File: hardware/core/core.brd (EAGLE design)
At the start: 161 x 144.8 mm, 520 parts, among them IC1 MAX481CSA, IC10 MAX481CSA, IC11 MAX481CSA, IC12 MAX481CSA, IC13 MAX481CSA, IC14 MAX481CSA, IC15 MAX481CSA, IC16 MAX481CSA, IC17 MAX481CSA, IC18 MAX481CSA, IC19 MAX481CSA, IC2 LD117AS12TR, IC20 MAX481CSA, IC21 MAX481CSA, IC22 LD117AS12TR, IC23 LD117AS12TR, IC3 MAX481CSA, IC4 MAX481CSA, IC5 MAX481CSA, IC6 MAX481CSA, IC7 MAX481CSA, IC8 MAX481CSA, IC9 MAX481CSA

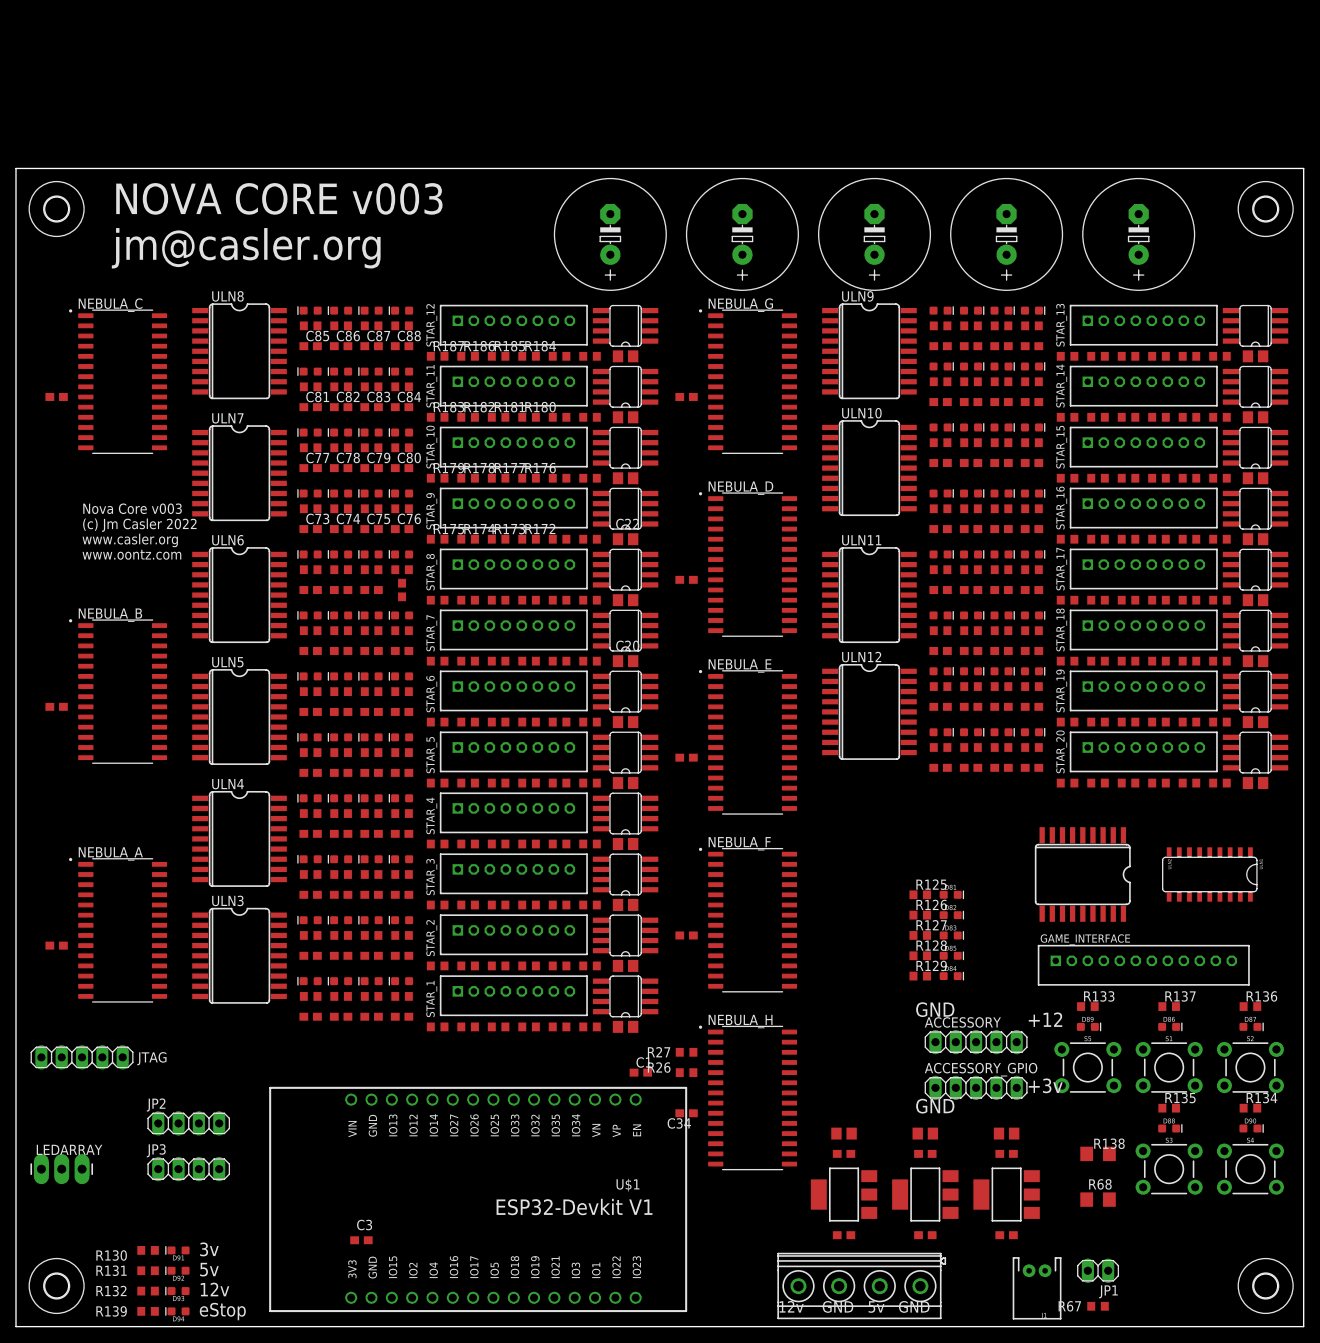
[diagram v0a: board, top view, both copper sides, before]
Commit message: Completed v3
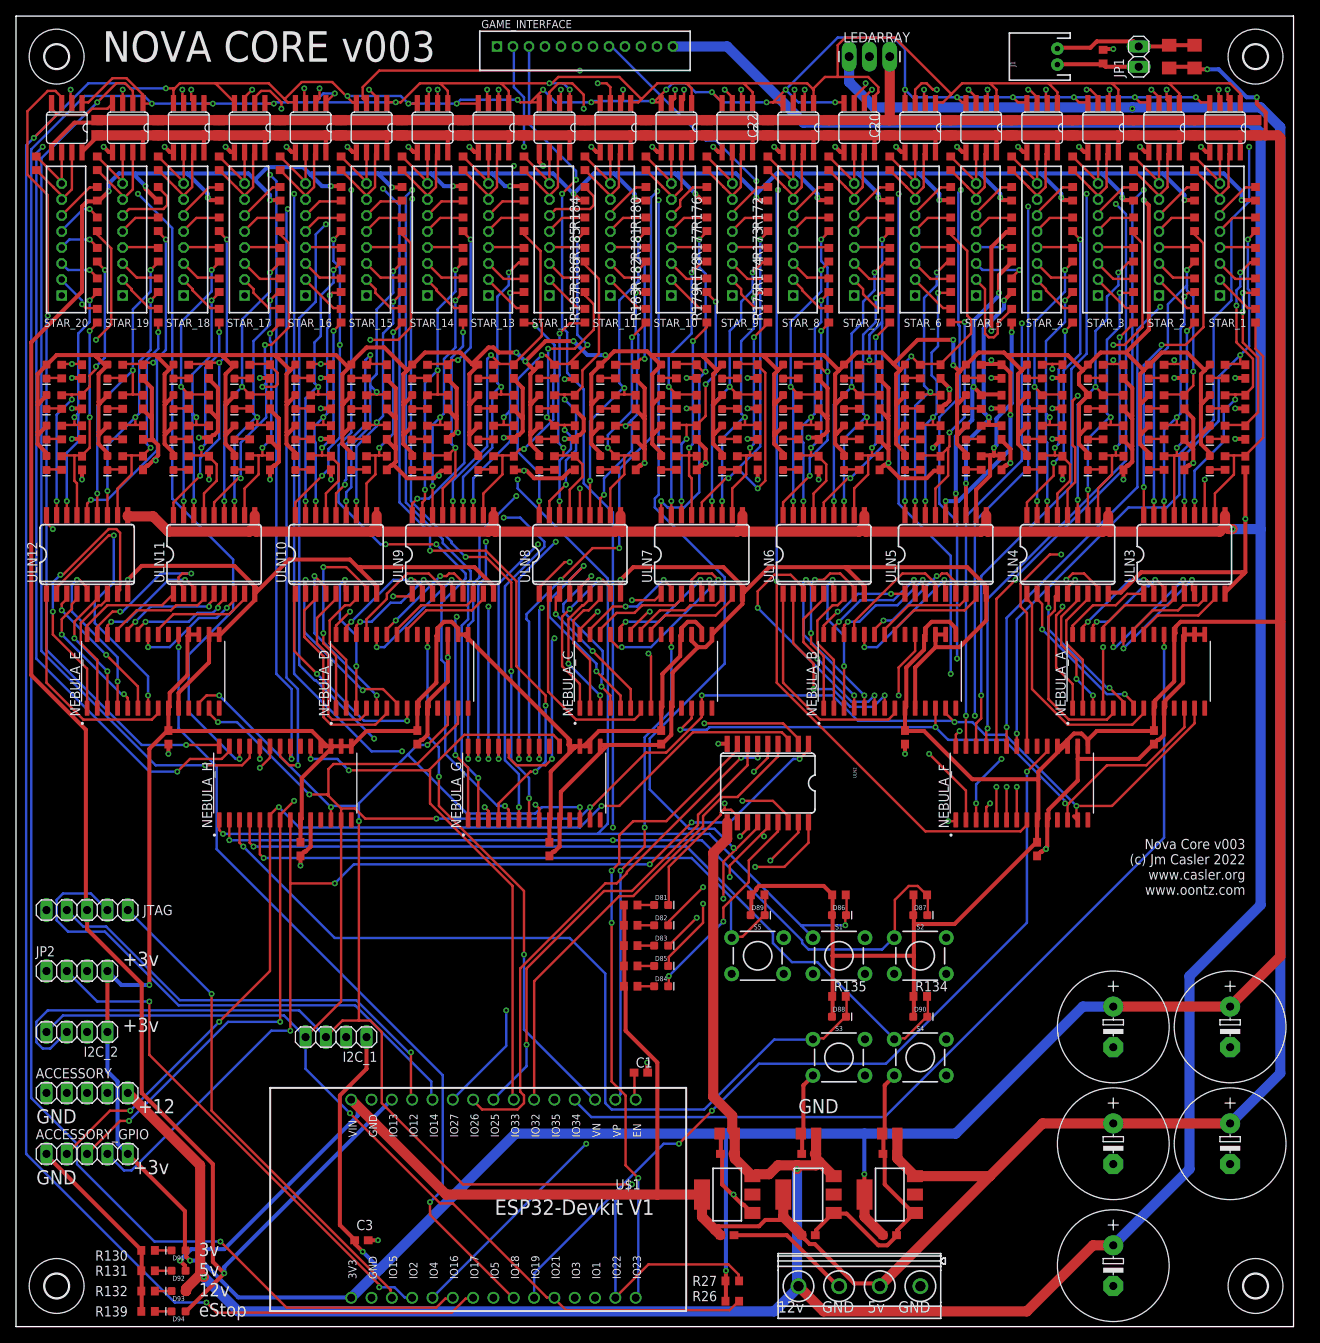
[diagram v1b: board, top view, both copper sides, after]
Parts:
- removed JP3: (no value), pinhead:1X04
- removed ULN1: (no value), SparkFun-IC-Special-Function:SO018
- added I2C_1, I2C_2: (no value), pinhead:1X04
- moved LEDARRAY 171.9 mm to (109.2, 158.8)
- moved IC21 167.9 mm to (6.35, 149.9), turned to 180 degrees
- moved R124 167.0 mm to (2.54, 145.4), turned to 270 degrees
- moved C26 166.3 mm to (10.2, 149.9), turned to 90 degrees
- moved IC20 157.6 mm to (14.0, 149.9), turned to 180 degrees
- moved R123 156.8 mm to (10.2, 145.4), turned to 270 degrees
- moved R67 156.2 mm to (135.9, 158.8), turned to 90 degrees
- moved C27 156.0 mm to (17.8, 149.9), turned to 90 degrees
- moved R106 155.1 mm to (10.2, 141.6), turned to 90 degrees
- moved JP1 151.8 mm to (140.3, 158.8), turned to 90 degrees
- moved J1 151.8 mm to (130.2, 158.8), turned to 90 degrees
- moved R216 150.0 mm to (10.2, 137.8), turned to 90 degrees
- moved STAR_20 149.4 mm to (5.71, 135.9), turned to 90 degrees
- moved IC19 147.4 mm to (21.6, 149.9), turned to 180 degrees
- moved R122 146.6 mm to (17.8, 145.4), turned to 270 degrees
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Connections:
- net +12V: no longer ULN1.10
- net +3V3: now also I2C_1.1, I2C_2.1; no longer JP3.1
- net 21/SDA: now also I2C_1.4, I2C_2.4; no longer JP3.4
- net 22/SCL: now also I2C_1.3, I2C_2.3; no longer JP3.3
- net 23: no longer ULN1.8
- net 25: no longer ULN1.7
- net 26: no longer ULN1.6
- net 27: no longer ULN1.5
- net 32: no longer ULN1.4
- net GND: now also I2C_1.2, I2C_2.2; no longer JP3.2, ULN1.9
- net H13: no longer ULN1.3
- net H14: no longer ULN1.2
- net H15: no longer ULN1.1
- net N$148: no longer ULN1.16
- net N$149: no longer ULN1.17
- net N$150: no longer ULN1.18
- net N$51: no longer ULN1.11
- net N$56: no longer ULN1.12
- net N$57: no longer ULN1.13
- net N$58: no longer ULN1.14
- net N$59: no longer ULN1.15
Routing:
- net +5V: track 0.00 -> 935.7 mm, vias 0 -> 9
- net +3V3: track 0.00 -> 926.9 mm, vias 0 -> 7
- net GND: track 0.00 -> 836.8 mm, vias 0 -> 77
- net +12V: track 0.00 -> 614.6 mm, vias 0 -> 3
- net 13: track 0.00 -> 454.0 mm, vias 0 -> 21
- net 16: track 0.00 -> 413.4 mm, vias 0 -> 8
- net 17: track 0.00 -> 409.2 mm, vias 0 -> 21
- net 22/SCL: track 0.00 -> 329.5 mm, vias 0 -> 9
- net 21/SDA: track 0.00 -> 315.1 mm, vias 0 -> 8
- net H10: track 0.00 -> 225.2 mm, vias 0 -> 1
- net H11: track 0.00 -> 218.3 mm, vias 0 -> 1
- net H9: track 0.00 -> 209.8 mm, vias 0 -> 5
- net H12: track 0.00 -> 196.2 mm, vias 0 -> 1
- net 4: track 0.00 -> 195.8 mm, vias 0 -> 1
- net H8: track 0.00 -> 195.2 mm, vias 0 -> 4
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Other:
- board size 161 x 144.8 mm -> 159.7 x 163.8 mm
- board text added: "NOVA CORE v003"
- board text removed: "NOVA CORE v003 jm@casler.org"
